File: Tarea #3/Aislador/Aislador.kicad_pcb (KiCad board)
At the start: 2 copper layers, 29 parts, among them IC1 ADUM5000ARWZ, IC2 NUP2202W1T2G, IC3 NUP2202W1T2G, IC4 ADUM4160BRWZ, J1 87520-0010BLF, J2 USB-B-S-F-B-TH-R

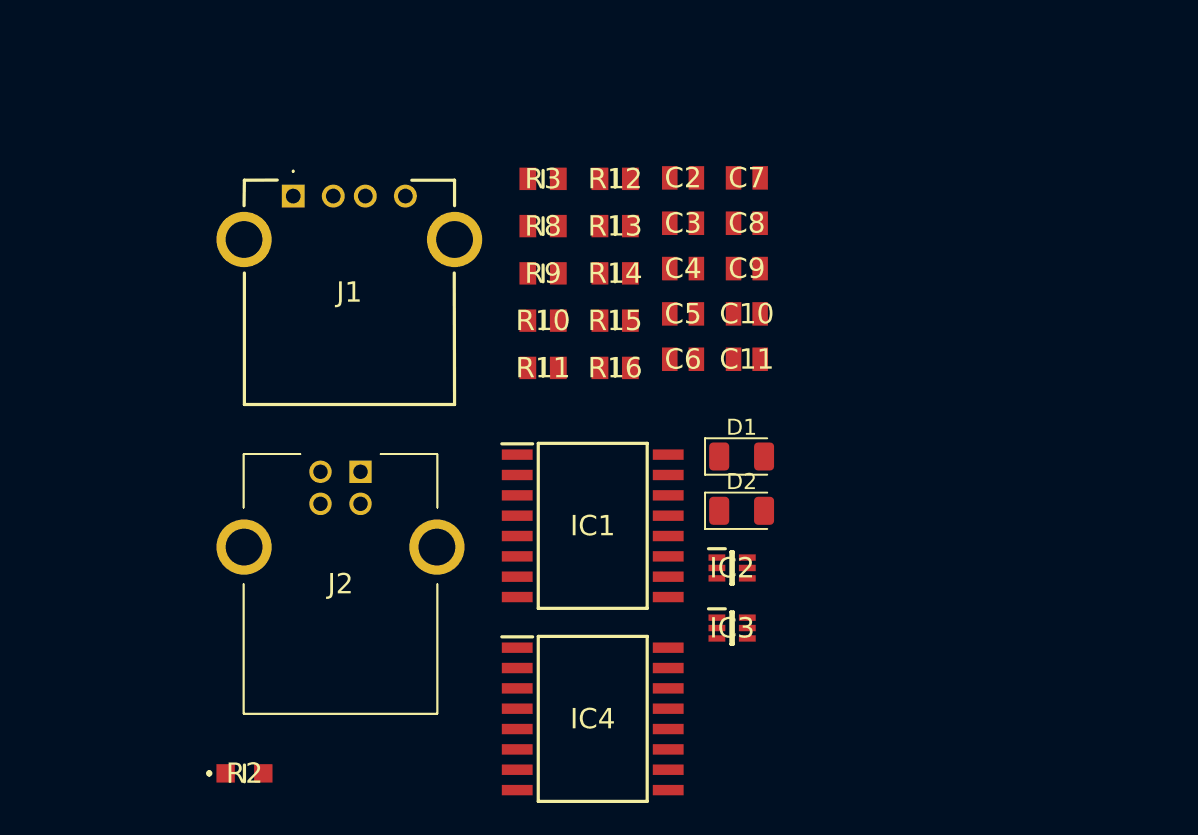
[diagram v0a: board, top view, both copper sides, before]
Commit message: Aislador
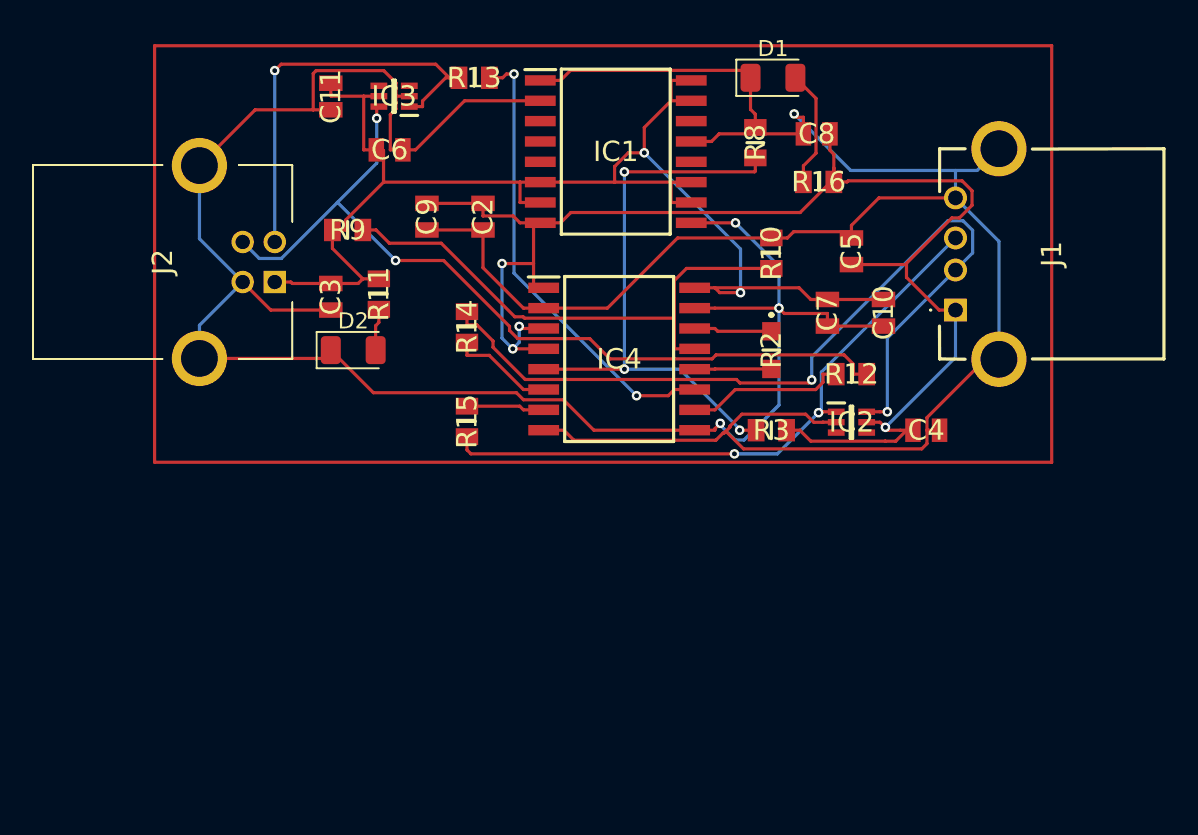
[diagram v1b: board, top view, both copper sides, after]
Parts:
- moved R2 42.2 mm to (167.5, 76.5), turned to -90 degrees
- moved J1 41.9 mm to (179.0, 74.0), turned to 90 degrees
- moved IC3 39.3 mm to (143.9, 60.6), turned to 180 degrees
- moved C11 30.7 mm to (140.0, 60.7), turned to -90 degrees
- moved D2 26.2 mm to (141.4, 76.5)
- moved D1 23.7 mm to (167.6, 59.5)
- moved IC1 23.4 mm to (157.8, 64.1)
- moved IC4 22.5 mm to (158.0, 77.1)
- moved C6 22.5 mm to (143.7, 64.0)
- moved C3 22.5 mm to (140.0, 73.2), turned to -90 degrees
- moved R3 21.2 mm to (167.5, 81.5), turned to 180 degrees
- moved C9 20.2 mm to (146.0, 68.2), turned to -90 degrees
- moved R12 19.1 mm to (172.5, 78.0)
- moved C4 18.2 mm to (177.2, 81.5)
- moved R16 17.2 mm to (170.4, 66.0), turned to 180 degrees
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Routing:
- net GND: track 0.00 -> 134.7 mm, vias 0 -> 1
- net GND1: track 0.00 -> 121.8 mm, vias 0 -> 3
- net +5V: track 0.00 -> 92.6 mm, vias 0 -> 4
- net VCC: track 0.00 -> 85.9 mm, vias 0 -> 2
- net /D-: track 0.00 -> 54.2 mm, vias 0 -> 2
- net /D5+: track 0.00 -> 53.0 mm, vias 0 -> 2
- net /D+: track 0.00 -> 39.5 mm, vias 0 -> 2
- net Net-(IC4-SPU): track 0.00 -> 36.2 mm, vias 0 -> 3
- net Net-(IC4-SPD): track 0.00 -> 33.6 mm
- net /D3-: track 0.00 -> 28.7 mm, vias 0 -> 2
- net /D5-: track 0.00 -> 26.2 mm, vias 0 -> 1
- net Net-(IC4-DD+): track 0.00 -> 10.1 mm
- net Net-(D1-A): track 0.00 -> 7.36 mm
- net /D2-: track 0.00 -> 6.50 mm
- net /D2+: track 0.00 -> 4.88 mm
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- added copper zone on B.Cu, net GND
- added copper zone on F.Cu, net GND
